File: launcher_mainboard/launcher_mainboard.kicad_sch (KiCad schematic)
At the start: 80 parts, among them J10 header, J11 header, J12 USB_C_Receptacle_USB2.0_16P, J2 Conn_01x06, J3 Conn_01x06, J4 Conn_01x06, J5 Conn_01x06, J6 bat_con, J7 fan_con, J8 ESC_1, J9 ESC_2, Q1 2N7002H, Q2 MMBT3904, Q3 MMBT3904, Q4 BSS138, Q5 BSS138, Q6 BSS138, Q7 BSS138, SW1 POWER_SWITCH, U10 TLV75533PDBV, U12 LM66200DRLR, U2 TMC2209-LA-T, U3 TMC2209-LA-T, U4 TMC2209-LA-T, U5 TMC2209-LA-T, U6 ESP32-S3-WROOM-1, U7 R-78E3.3-0.5, U8 D3V3XA4B10LP, U9 R-78E5.0-0.5

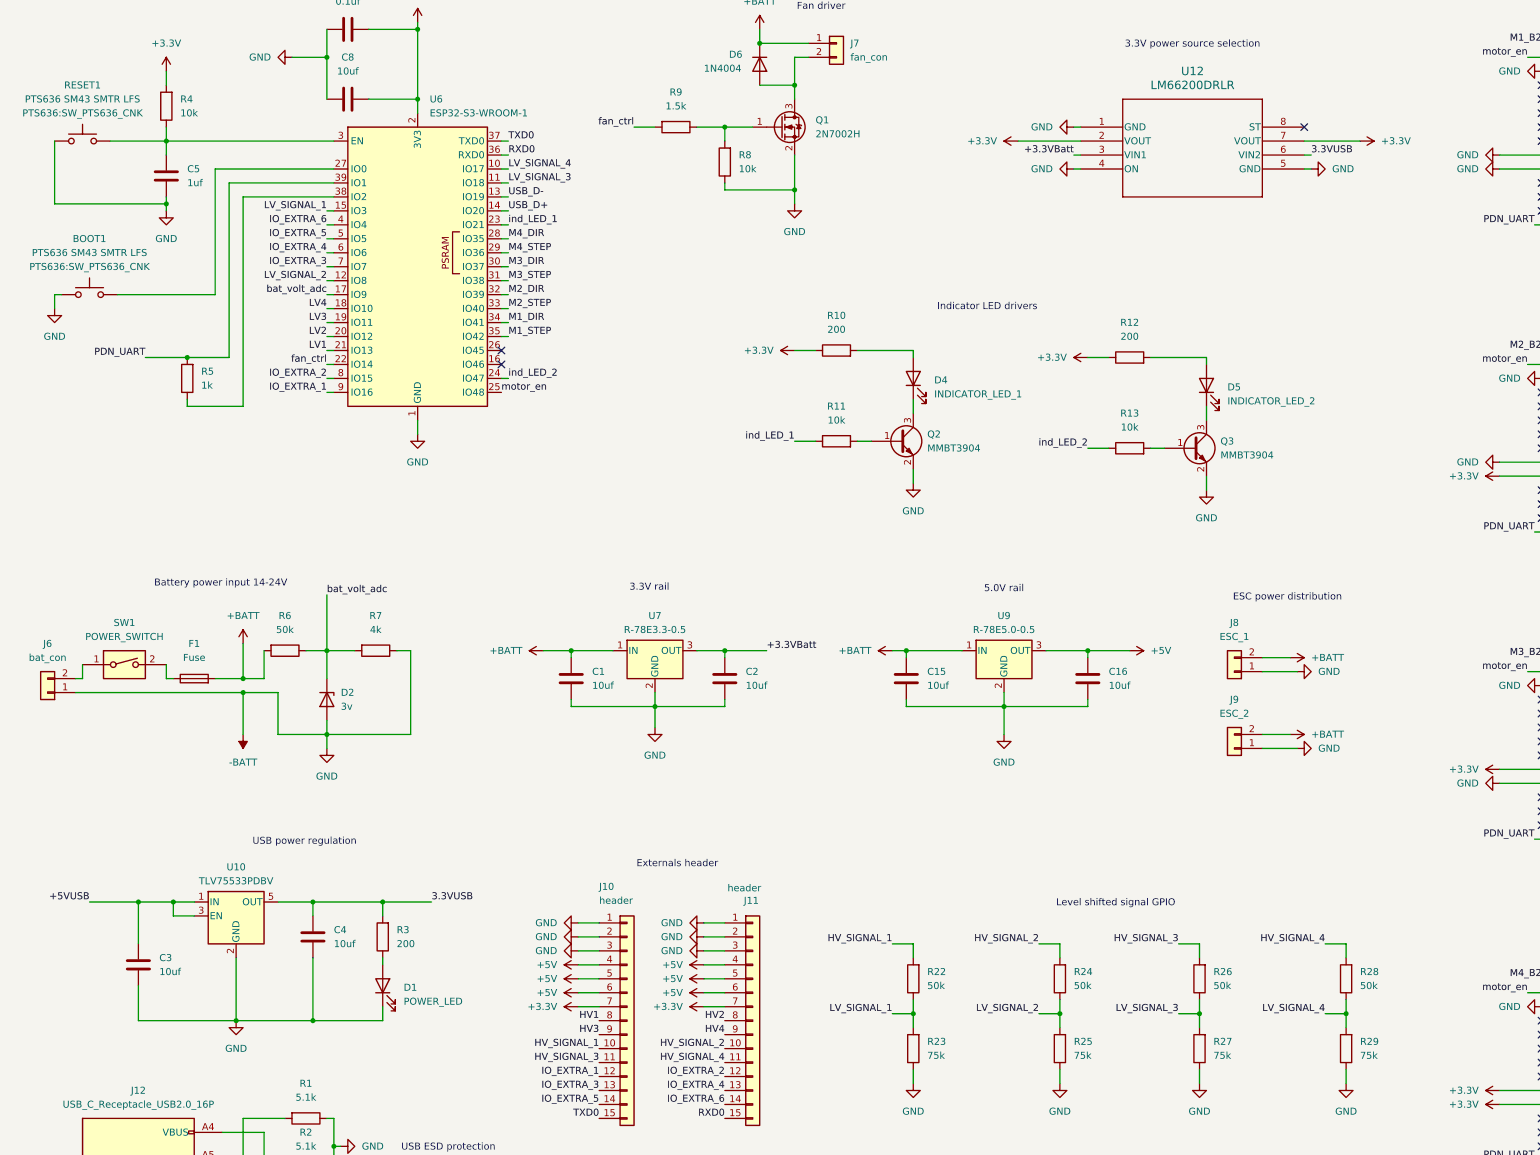
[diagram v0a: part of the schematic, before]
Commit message: more layout
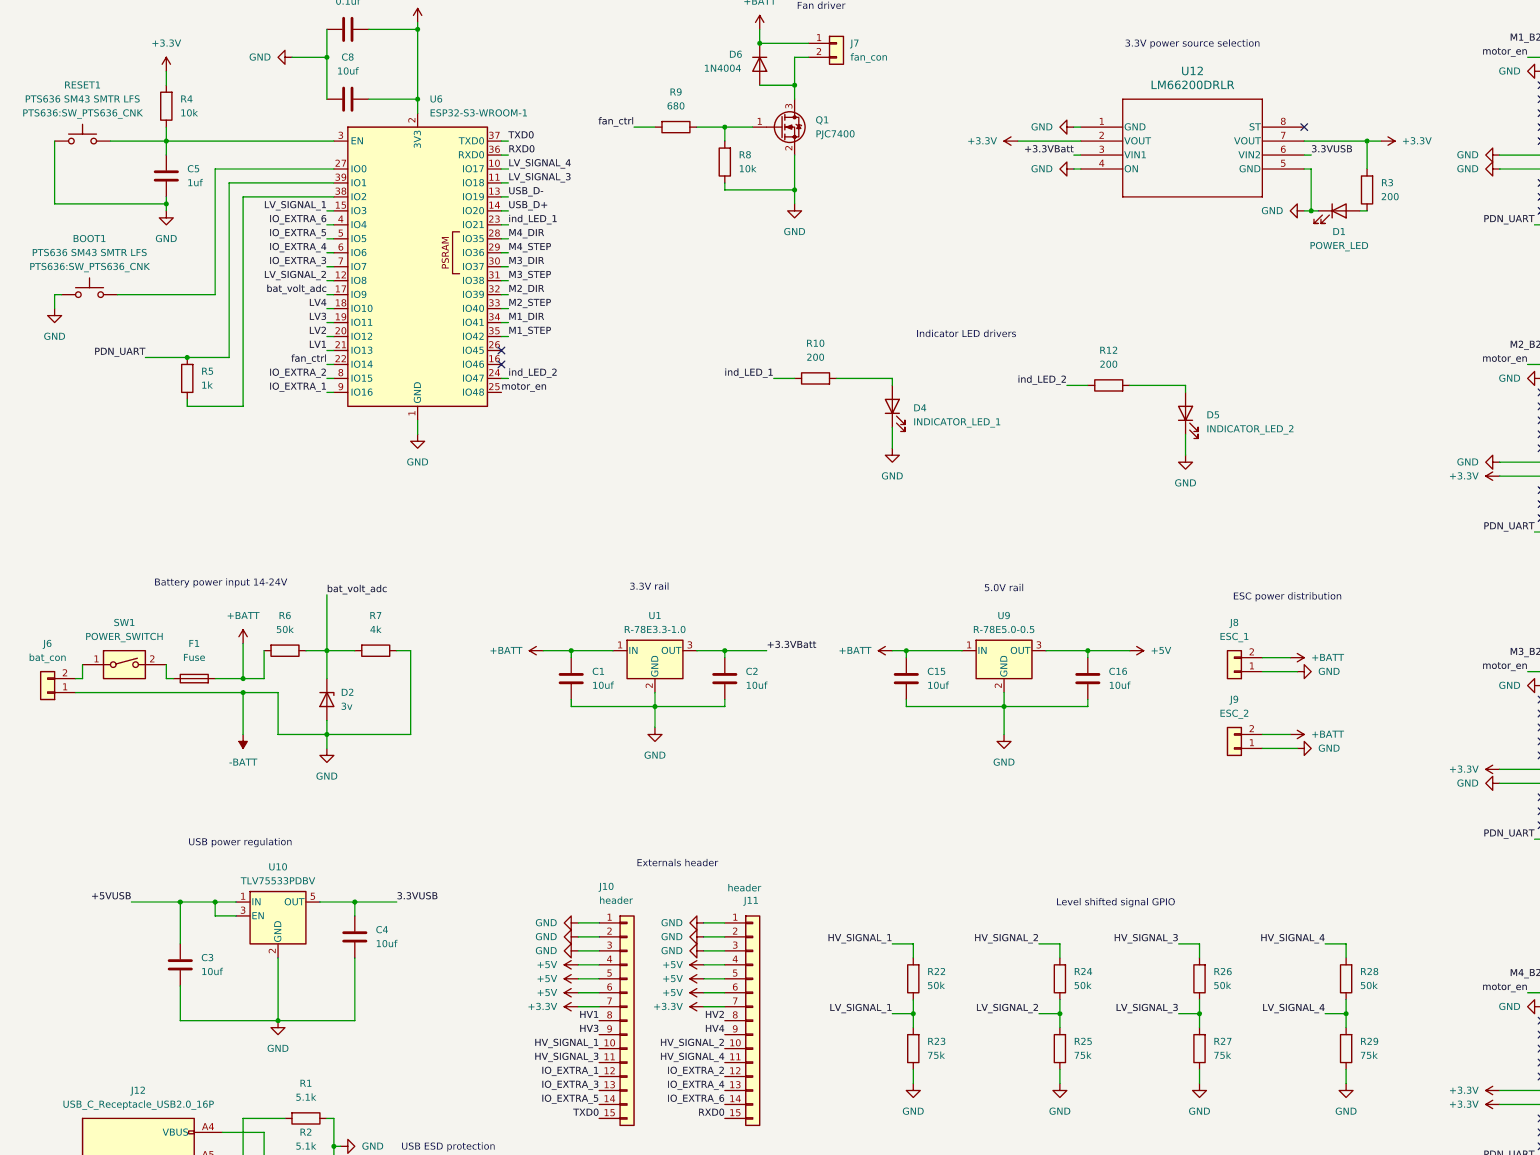
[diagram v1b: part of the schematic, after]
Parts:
- removed Q2, Q3: MMBT3904, Package_TO_SOT_SMD:SOT-23, symbol Transistor_BJT:MMBT3904
- removed R11, R13: 10k, Resistor_SMD:R_0805_2012Metric, symbol Device:R
- removed U7: R-78E3.3-0.5, Converter_DCDC:Converter_DCDC_RECOM_R-78E-0.5_THT, symbol Regulator_Switching:R-78E3.3-0.5
- added U1: R-78E3.3-1.0, Converter_DCDC:Converter_DCDC_RECOM_R-78E-0.5_THT, symbol Regulator_Switching:R-78E3.3-1.0
- D1, D4, D5: footprint LED_SMD:LED_PLCC-2_3x2mm_AK -> LED_SMD:LED_0805_2012Metric
- D2: footprint Diode_SMD:D_0201_0603Metric -> Diode_SMD:D_0805_2012Metric
- D6: footprint Diode_THT:D_DO-35_SOD27_P5.08mm_Vertical_KathodeUp -> Diode_SMD:D_0805_2012Metric
- J7: footprint Connector_Molex:Molex_PicoBlade_53047-0210_1x02_P1.25mm_Vertical -> Connector_JST:JST_XH_B2B-XH-A_1x02_P2.50mm_Vertical
- Q1: value 2N7002H -> PJC7400; footprint Package_TO_SOT_SMD:SOT-23 -> Package_TO_SOT_SMD:SOT-323_SC-70
- R9: value 1.5k -> 680
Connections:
- net +3.3V: now also R3.2; no longer R10.1, R12.1
- net +3.3VBatt: now also U1.3 (OUT)
- net +BATT: now also U1.1 (IN)
- net -BATT: now also D4.1 (K), D5.1 (K), U1.2 (GND)
- net 3.3VUSB: no longer R3.2
- net ind_LED_1: now also R10.1
- net ind_LED_2: now also R12.1
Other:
- moved on the sheet: C3, C4, D1, D4, D5, R10, R12, R3, U10
